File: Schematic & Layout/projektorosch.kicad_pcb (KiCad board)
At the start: 2 copper layers, 92.3 x 67.8 mm, 24 parts, among them J1 Barrel_Jack_Switch, J2 Conn_01x03, J3 RJ12, U1 ATtiny3216-S, U2 MAX232

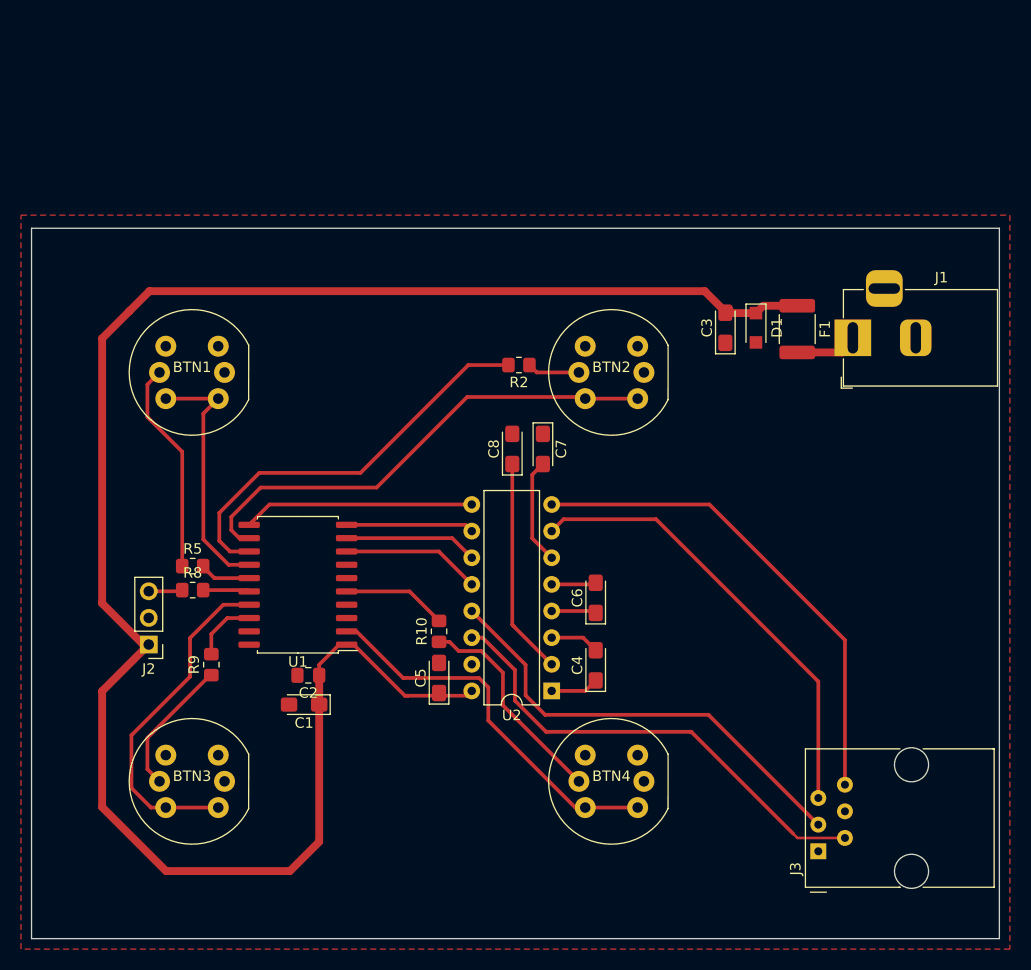
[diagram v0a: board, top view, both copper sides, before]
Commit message: SEM ProjektoroSCH Revision 2
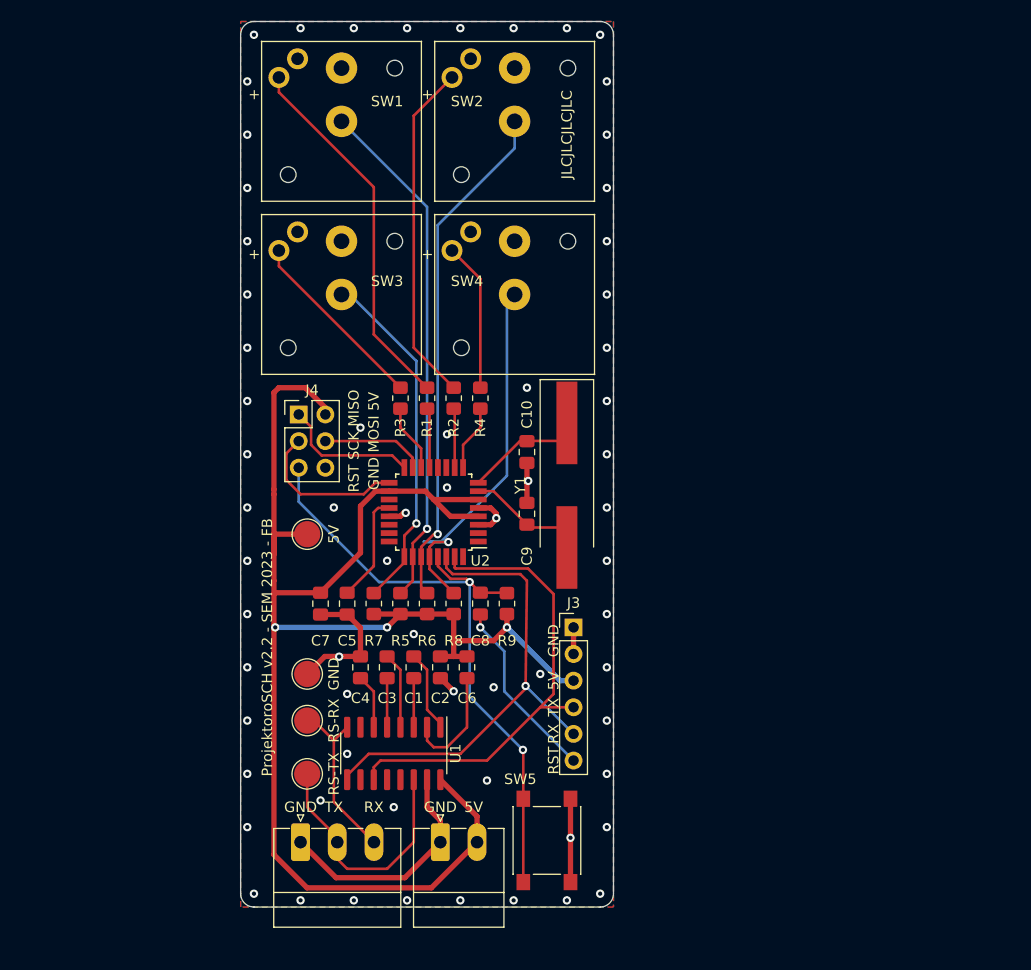
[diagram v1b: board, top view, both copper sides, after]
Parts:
- removed BTN1, BTN2, BTN3, BTN4: LEDBTN, ledbtn_footprint:LBTN
- removed D1: D_Zener 5.6V, Diode_SMD:Nexperia_CFP3_SOD-123W
- removed F1: Polyfuse, Fuse:Fuse_1812_4532Metric_Pad1.30x3.40mm_HandSolder
- removed R10: 220R, Resistor_SMD:R_0805_2012Metric_Pad1.20x1.40mm_HandSolder
- added 5V: 5V, TestPoint:TestPoint_Pad_D2.5mm, F.Cu at (134.0, 98.4)
- added C10: 22pF, Capacitor_SMD:C_0805_2012Metric_Pad1.18x1.45mm_HandSolder, F.Cu at (154.9, 90.6)
- added C9: 22pF, Capacitor_SMD:C_0805_2012Metric_Pad1.18x1.45mm_HandSolder, F.Cu at (154.9, 96.5)
- added GND: GND, TestPoint:TestPoint_Pad_D2.5mm, F.Cu at (134.0, 111.8)
- added J4: ISP, Connector_PinHeader_2.54mm:PinHeader_2x03_P2.54mm_Vertical, F.Cu at (133.2, 87.0)
- added R1: 150, Resistor_SMD:R_0805_2012Metric_Pad1.20x1.40mm_HandSolder, F.Cu at (145.4, 85.5)
- added R3: 150, Resistor_SMD:R_0805_2012Metric_Pad1.20x1.40mm_HandSolder, F.Cu at (142.9, 85.5)
- added R4: 150, Resistor_SMD:R_0805_2012Metric_Pad1.20x1.40mm_HandSolder, F.Cu at (150.5, 85.5)
- added R6: 10k, Resistor_SMD:R_0805_2012Metric_Pad1.20x1.40mm_HandSolder, F.Cu at (145.4, 105.0)
- added R7: 10k, Resistor_SMD:R_0805_2012Metric_Pad1.20x1.40mm_HandSolder, F.Cu at (140.3, 105.0)
- added RS-RX: 232-RX, TestPoint:TestPoint_Pad_D2.5mm, F.Cu at (134.0, 116.2)
- added RS-TX: 232-TX, TestPoint:TestPoint_Pad_D2.5mm, F.Cu at (134.0, 121.3)
- added SW1: SW_SPST, Library:Marquardt 64250101, F.Cu at (137.3, 59.1)
- added SW2: SW_SPST, Library:Marquardt 64250101, F.Cu at (153.8, 59.1)
- added SW3: SW_SPST, Library:Marquardt 64250101, F.Cu at (137.3, 75.6)
- added SW4: SW_SPST, Library:Marquardt 64250101, F.Cu at (153.8, 75.6)
- added SW5: Reset, Button_Switch_SMD:SW_Push_1P1T_NO_6x6mm_H9.5mm, F.Cu at (156.8, 127.6)
- added Y1: 16MHz, Crystal:Crystal_SMD_HC49-SD_HandSoldering, F.Cu at (158.8, 93.8)
- C1, C4, C5, C6, C7, C8: value 1u -> 0.1uF; footprint Capacitor_Tantalum_SMD:CP_EIA-3216-10_Kemet-I_Pad1.58x1.35mm_HandSolder -> Capacitor_SMD:C_0805_2012Metric_Pad1.18x1.45mm_HandSolder
- C2: value 100n -> 0.1uF
- C3: value 10uF -> 0.1uF; footprint Capacitor_Tantalum_SMD:CP_EIA-3216-12_Kemet-S_Pad1.58x1.35mm_HandSolder -> Capacitor_SMD:C_0805_2012Metric_Pad1.18x1.45mm_HandSolder
- J1: value Barrel_Jack_Switch -> Power; footprint Connector_BarrelJack:BarrelJack_Horizontal -> Connector_Phoenix_MC:PhoenixContact_MC_1,5_2-G-3.5_1x02_P3.50mm_Horizontal
- J2: value Conn_01x03 -> RS232; footprint Connector_PinHeader_2.54mm:PinHeader_1x03_P2.54mm_Vertical -> Connector_Phoenix_MC:PhoenixContact_MC_1,5_3-G-3.5_1x03_P3.50mm_Horizontal
- J3: value RJ12 -> Programmer; footprint Connector_RJ:RJ12_Amphenol_54601 -> Connector_PinHeader_2.54mm:PinHeader_1x06_P2.54mm_Vertical
- R2: value 220R -> 150
- R5, R9: value 220R -> 10k
- R8: value 470R -> 10k
- U1: value ATtiny3216-S -> MAX232; footprint Package_SO:SOIC-20W_7.5x12.8mm_P1.27mm -> Package_SO:SOP-16_3.9x9.9mm_P1.27mm
- U2: value MAX232 -> ATmega328P-A; footprint Package_DIP:DIP-16_W7.62mm -> Package_QFP:TQFP-32_7x7mm_P0.8mm
- moved J1 62.1 mm to (146.7, 127.8), turned to 0 degrees
- moved C3 45.7 mm to (141.6, 111.1), turned to -90 degrees
- moved J3 31.6 mm to (159.4, 107.3), turned to 0 degrees
- moved R9 28.8 mm to (153.0, 105.0), turned to -90 degrees
- moved C7 25.8 mm to (135.3, 105.1), turned to 90 degrees
- moved R8 24.9 mm to (148.0, 105.0), turned to -90 degrees
- moved J2 23.8 mm to (133.3, 127.8), turned to 0 degrees
- moved C4 22.4 mm to (139.1, 111.1), turned to -90 degrees
- moved U2 20.4 mm to (146.1, 96.3)
- moved R5 20.1 mm to (142.9, 105.0), turned to -90 degrees
- moved U1 18.5 mm to (142.2, 119.3), turned to -90 degrees
- moved C8 15.1 mm to (150.5, 105.0), turned to -90 degrees
- moved C6 13.9 mm to (149.2, 111.1)
- moved C2 12.6 mm to (146.7, 111.1), turned to -90 degrees
- moved C5 11.3 mm to (137.8, 105.1)
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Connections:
- C1 pad 1: VCC -> Net-(U1-C1+)
- C1 pad 2: GND -> Net-(U1-C1-)
- C2 pad 1: VCC -> +5V
- C3 pad 1: GND -> Net-(U1-C2+)
- C3 pad 2: VCC -> Net-(U1-C2-)
- C4 pad 1: Net-(C4-Pad1) -> GND
- C4 pad 2: Net-(C4-Pad2) -> Net-(U1-VS-)
- C5 pad 1: VCC -> GND
- C5 pad 2: GND -> Net-(U2-AREF)
- C6 pad 1: Net-(C6-Pad1) -> Net-(U1-VS+)
- C6 pad 2: Net-(C6-Pad2) -> +5V
- C7 pad 2: Net-(C7-Pad2) -> +5V
- C8 pad 1: Net-(C8-Pad1) -> RST
- C8 pad 2: GND -> PROG-DTR
- J1 pad 1: Net-(F1-Pad2) -> GND
- J1 pad 2: GND -> +5V
- J2 pad 1: VCC -> GND
- J2 pad 2: GND -> 232-TX
- J2 pad 3: Net-(J2-Pad3) -> 232-RX
- J3 pad 2: TX -> GND
- J3 pad 3: RX -> +5V
- J3 pad 4: unconnected-(J3-Pad4) -> MCU-TX
- J3 pad 5: CTS -> MCU-RX
- J3 pad 6: RTS -> PROG-DTR
- R2 pad 2: BTN2LED -> PWM-2
- R5 pad 1: Net-(BTN1-Pad3) -> BTN-1
- R5 pad 2: BTN1LED -> +5V
- R8 pad 1: Net-(J2-Pad3) -> BTN-4
- R8 pad 2: UPDI -> +5V
- R9 pad 1: Net-(BTN3-Pad3) -> RST
- R9 pad 2: BTN3LED -> +5V
- U1 pad 1: VCC -> Net-(U1-C1+)
- U1 pad 10: CTSD -> unconnected-(U1-T2IN-Pad10)
- U1 pad 11: RTSD -> MCU-TX
- U1 pad 12: BTN2 -> unconnected-(U1-R1OUT-Pad12)
- U1 pad 13: BTN2LED -> unconnected-(U1-R1IN-Pad13)
- U1 pad 14: BTN1 -> 232-TX
- U1 pad 15: BTN1LED -> GND
- U1 pad 16: UPDI -> +5V
- U1 pad 2: BTN4 -> Net-(U1-VS+)
- U1 pad 3: GND -> Net-(U1-C1-)
- U1 pad 4: GND -> Net-(U1-C2+)
- U1 pad 5: BTN4LED -> Net-(U1-C2-)
- U1 pad 6: unconnected-(U1-Pad6) -> Net-(U1-VS-)
- U1 pad 8: RXD -> 232-RX
- U1 pad 9: TXD -> MCU-RX
- U2 pad 1: Net-(C4-Pad1) -> unconnected-(U2-PD3-Pad1)
- U2 pad 10: CTSD -> PWM-2
- U2 pad 11: TXD -> unconnected-(U2-PD7-Pad11)
- U2 pad 12: RXD -> unconnected-(U2-PB0-Pad12)
- U2 pad 13: RX -> PWM-1
- U2 pad 14: TX -> PWM-3
- U2 pad 15: GND -> MOSI
- U2 pad 16: VCC -> MISO
- U2 pad 2: Net-(C8-Pad1) -> unconnected-(U2-PD4-Pad2)
- U2 pad 3: Net-(C4-Pad2) -> GND
- U2 pad 4: Net-(C6-Pad1) -> +5V
- U2 pad 5: Net-(C6-Pad2) -> GND
- U2 pad 6: Net-(C7-Pad2) -> +5V
- U2 pad 7: CTS -> Net-(U2-XTAL1/PB6)
- U2 pad 8: RTS -> Net-(U2-XTAL2/PB7)
- U2 pad 9: RTSD -> PWM-4
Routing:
- net VCC: track 177.1 -> 0.00 mm
- net +5V: track 0.00 -> 159.1 mm, vias 0 -> 3
- net RST: track 0.00 -> 62.0 mm, vias 0 -> 2
- net GND: track 0.00 -> 58.5 mm, vias 0 -> 66
- net BTN-1: track 0.00 -> 49.4 mm, vias 0 -> 1
- net BTN-2: track 0.00 -> 49.1 mm, vias 0 -> 1
- net RTS: track 47.1 -> 0.00 mm
- net MCU-RX: track 0.00 -> 47.0 mm, vias 0 -> 1
- net BTN2: track 46.8 -> 0.00 mm
- net MCU-TX: track 0.00 -> 45.5 mm
- net TX: track 45.2 -> 0.00 mm
- net CTS: track 43.4 -> 0.00 mm
- net RX: track 43.2 -> 0.00 mm
- net BTN2LED: track 39.3 -> 0.00 mm
- net BTN-4: track 0.00 -> 37.8 mm, vias 0 -> 1
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- added copper zone on B.Cu, net GND
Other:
- board size 92.3 x 67.8 mm -> 35.6 x 84.5 mm
